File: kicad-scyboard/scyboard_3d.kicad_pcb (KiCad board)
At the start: 2 copper layers, 144 x 96.5 mm, 55 parts

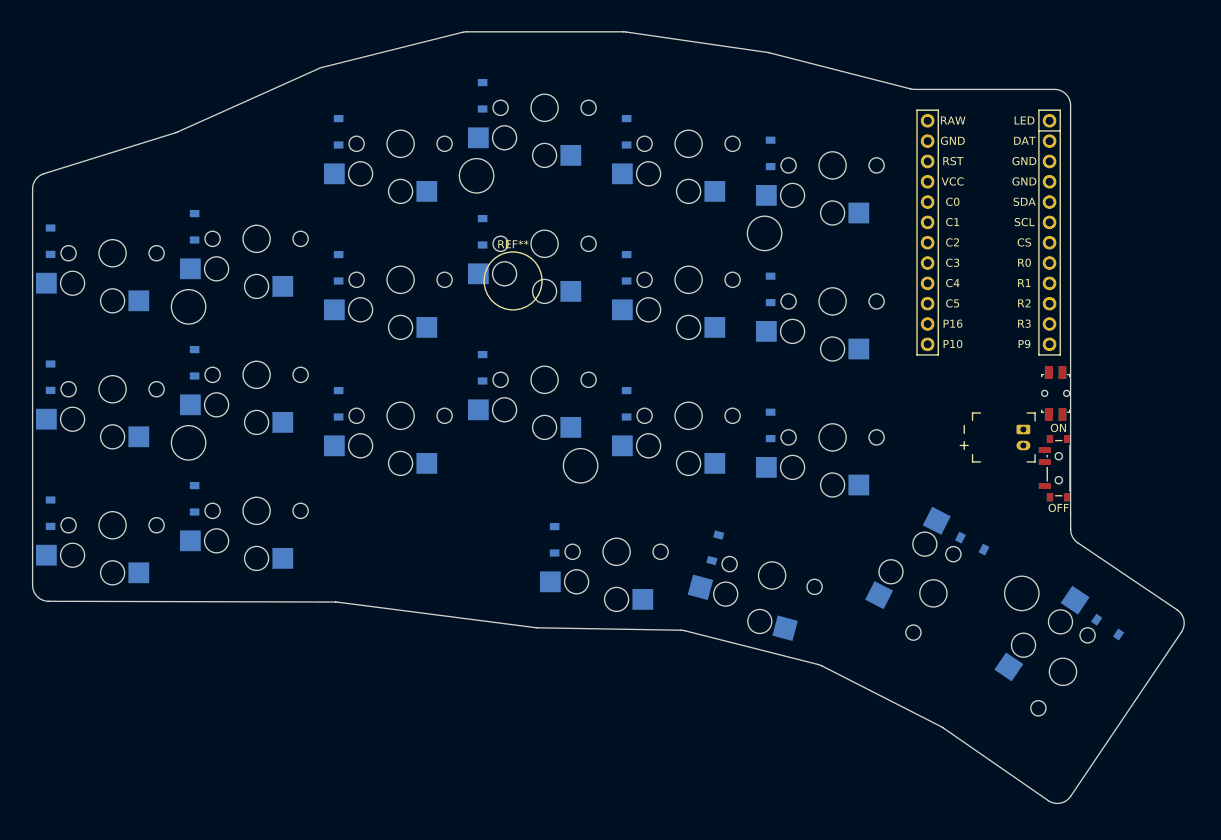
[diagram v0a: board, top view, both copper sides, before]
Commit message: Compile
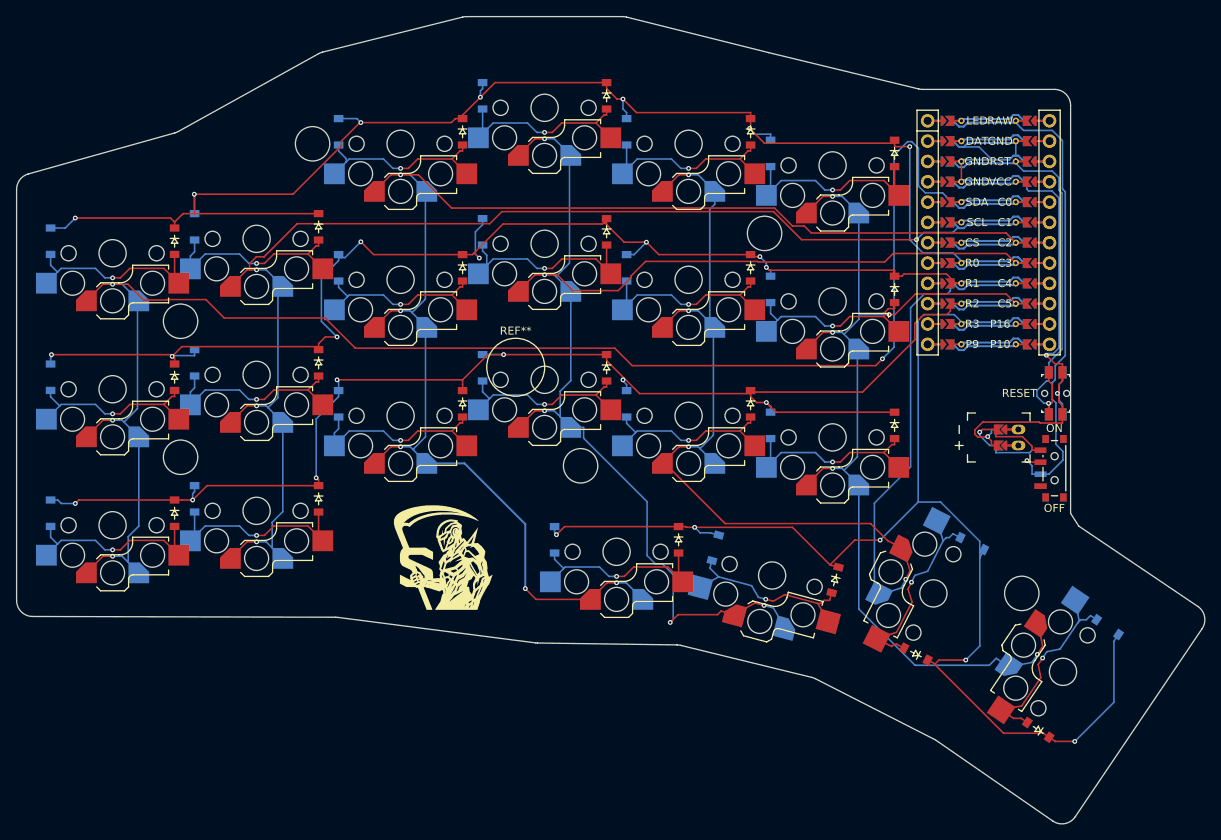
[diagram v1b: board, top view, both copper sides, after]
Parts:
- added D23: , ceoloide:diode_tht_sod123, F.Cu at (57.8, 98.5)
- added D24: , ceoloide:diode_tht_sod123, F.Cu at (57.8, 81.5)
- added D25: , ceoloide:diode_tht_sod123, F.Cu at (57.8, 64.5)
- added D26: , ceoloide:diode_tht_sod123, F.Cu at (75.8, 96.7)
- added D27: , ceoloide:diode_tht_sod123, F.Cu at (75.8, 79.7)
- added D28: , ceoloide:diode_tht_sod123, F.Cu at (75.8, 62.7)
- added D29: , ceoloide:diode_tht_sod123, F.Cu at (93.8, 84.8)
- added D30: , ceoloide:diode_tht_sod123, F.Cu at (93.8, 67.8)
- added D31: , ceoloide:diode_tht_sod123, F.Cu at (93.8, 50.8)
- added D32: , ceoloide:diode_tht_sod123, F.Cu at (111.8, 80.3)
- added D33: , ceoloide:diode_tht_sod123, F.Cu at (111.8, 63.3)
- added D34: , ceoloide:diode_tht_sod123, F.Cu at (111.8, 46.3)
- added D35: , ceoloide:diode_tht_sod123, F.Cu at (129.8, 84.8)
- added D36: , ceoloide:diode_tht_sod123, F.Cu at (129.8, 67.8)
- added D37: , ceoloide:diode_tht_sod123, F.Cu at (129.8, 50.8)
- added D38: , ceoloide:diode_tht_sod123, F.Cu at (147.8, 87.5)
- added D39: , ceoloide:diode_tht_sod123, F.Cu at (147.8, 70.5)
- added D40: , ceoloide:diode_tht_sod123, F.Cu at (147.8, 53.5)
- added D41: , ceoloide:diode_tht_sod123, F.Cu at (120.8, 101.8)
- added D42: , ceoloide:diode_tht_sod123, F.Cu at (140.3, 106.8)
- added D43: , ceoloide:diode_tht_sod123, F.Cu at (150.4, 116.1)
- added D44: , ceoloide:diode_tht_sod123, F.Cu at (165.7, 125.6)
- added G***: LOGO, custom:scyboard_logo, F.Cu at (91.1, 104.1)
- JST1: footprint custom:custom_battery_connector_jst_ph_2 -> custom:custom_reversible_battery_connector_jst_ph_2
- MCU1: footprint ceoloide:mcu_nice_nano -> custom:custom_reversible_mcu_nice_nano_flipped
- MH3: footprint custom:custom_mounting_hole_npth_loose -> custom:custom_mounting_hole_npth_tight
- PWR1: footprint custom:custom_power_switch_smd_side -> custom:custom_reversible_power_switch_smd_side
- RST1: footprint custom:custom_reset_switch_smd_side -> custom:custom_reversible_reset_switch_smd_side
- S1, S10, S11, S12, S13, S14, S15, S16, S17, S18, S19, S2, S20, S3, S4, S5, S6, S7, S8, S9: footprint custom:custom_switch_choc_v1 -> custom:custom_reversible_switch_choc_v1_oneside
- S21: footprint custom:custom_switch_choc_v1_1.5u -> custom:custom_reversible_switch_choc_v1_oneside
- S22: footprint custom:custom_switch_choc_v1 -> custom:custom_reversible_switch_choc_v1_oneside_1.5u
- moved MH6 57.4 mm to (108.5, 92.6)
- moved MH5 55.3 mm to (163.7, 108.5)
- moved MH3 52.4 mm to (75.0, 52.3)
- moved MH4 36.7 mm to (131.5, 63.5)
- moved REF** 10.8 mm to (100.4, 80.2)
- moved MH1 2.06 mm to (58.5, 74.5)
- moved MH2 2.06 mm to (58.5, 91.5)
- moved JST1 0.62 mm to (163.2, 89.0)
- moved PWR1 0.53 mm to (167.7, 92.9)
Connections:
- JST1 pad 1: GND -> BAT_P
- JST1 pad 2: BAT_P -> GND
- MCU1 pad 1: LED -> MCU1_1
- MCU1 pad 10: R2 -> MCU1_10
- MCU1 pad 11: R3 -> MCU1_11
- MCU1 pad 12: P9 -> MCU1_12
- MCU1 pad 13: P10 -> MCU1_13
- MCU1 pad 14: P16 -> MCU1_14
- MCU1 pad 15: C5 -> MCU1_15
- MCU1 pad 16: C4 -> MCU1_16
- MCU1 pad 17: C3 -> MCU1_17
- MCU1 pad 18: C2 -> MCU1_18
- MCU1 pad 19: C1 -> MCU1_19
- MCU1 pad 2: DAT -> MCU1_2
- MCU1 pad 20: C0 -> MCU1_20
- MCU1 pad 21: VCC -> MCU1_21
- MCU1 pad 22: RST -> MCU1_22
- MCU1 pad 23: GND -> MCU1_23
- MCU1 pad 24: RAW -> MCU1_24
- MCU1 pad 3: GND -> MCU1_3
- MCU1 pad 4: GND -> MCU1_4
- MCU1 pad 5: SDA -> MCU1_5
- MCU1 pad 6: SCL -> MCU1_6
- MCU1 pad 7: CS -> MCU1_7
- MCU1 pad 8: R0 -> MCU1_8
- MCU1 pad 9: R1 -> MCU1_9
- PWR1 pad 1: (no net) -> BAT_P
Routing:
- net C0: track 0.00 -> 207.9 mm, vias 0 -> 4
- net C2: track 0.00 -> 188.3 mm, vias 0 -> 5
- net R0: track 0.00 -> 182.8 mm, vias 0 -> 7
- net C3: track 0.00 -> 177.8 mm, vias 0 -> 5
- net R2: track 0.00 -> 174.8 mm, vias 0 -> 7
- net R3: track 0.00 -> 164.1 mm, vias 0 -> 5
- net R1: track 0.00 -> 161.6 mm, vias 0 -> 8
- net C1: track 0.00 -> 161.6 mm, vias 0 -> 4
- net C4: track 0.00 -> 156.5 mm, vias 0 -> 4
- net C5: track 0.00 -> 135.1 mm, vias 0 -> 5
- net GND: track 0.00 -> 98.2 mm, vias 0 -> 3
- net RAW: track 0.00 -> 67.0 mm, vias 0 -> 1
- net RST: track 0.00 -> 55.4 mm, vias 0 -> 1
- net space_cluster_B: track 0.00 -> 27.6 mm, vias 0 -> 1
- net reach_cluster_B: track 0.00 -> 25.7 mm, vias 0 -> 1
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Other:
- board size 144 x 96.5 mm -> 148.5 x 100.9 mm
